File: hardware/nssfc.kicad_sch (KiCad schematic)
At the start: 27 parts, among them U1 STM32F405RGTx, U2 W25Q128JVP, U3 QMC5883P, U4 ICM-20602, U5 BMP580, Y1 25MHz

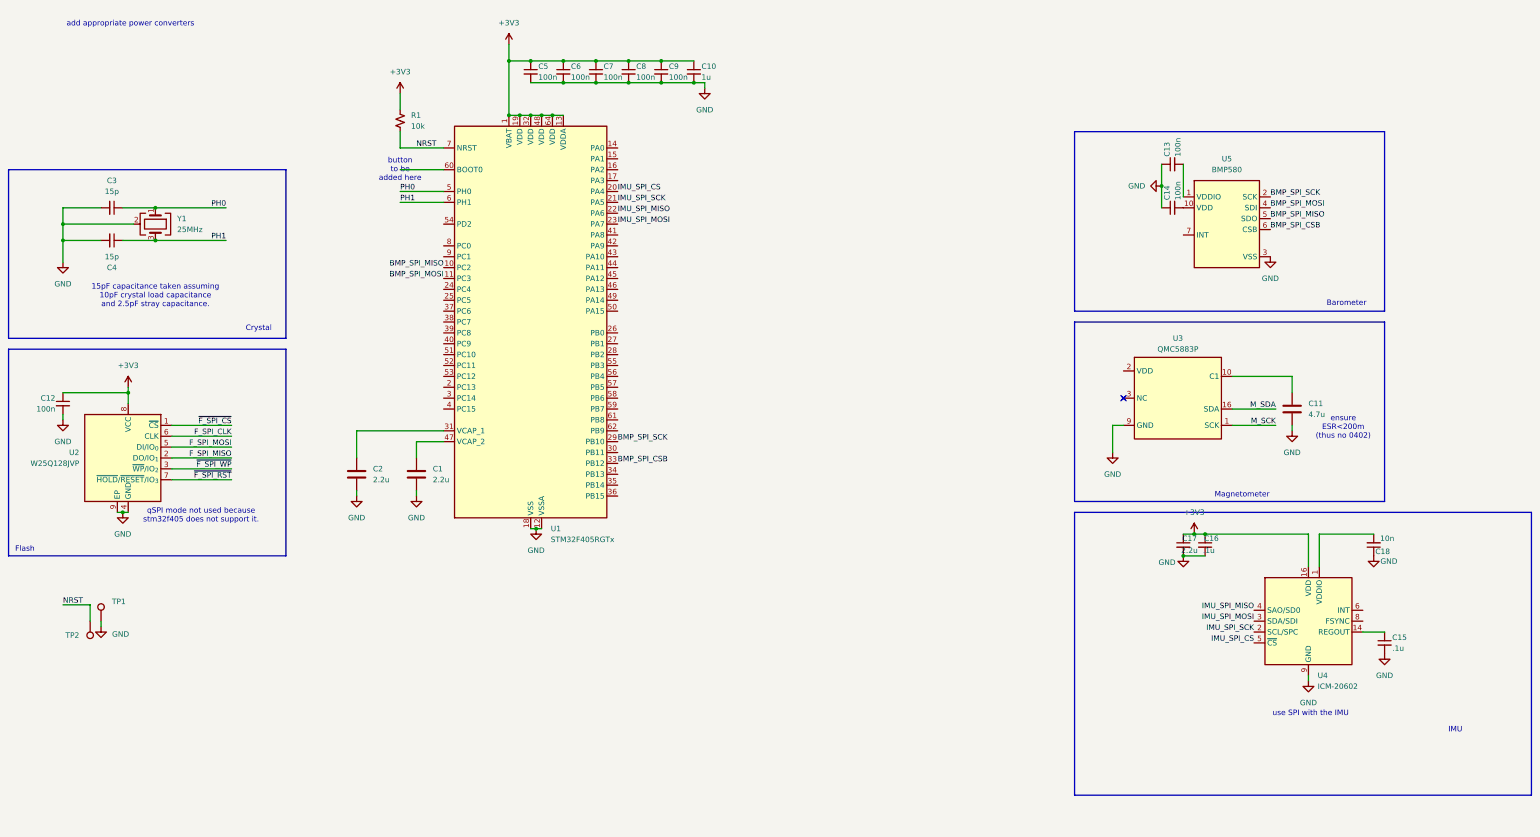
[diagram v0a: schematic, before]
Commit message: worked on the schematic
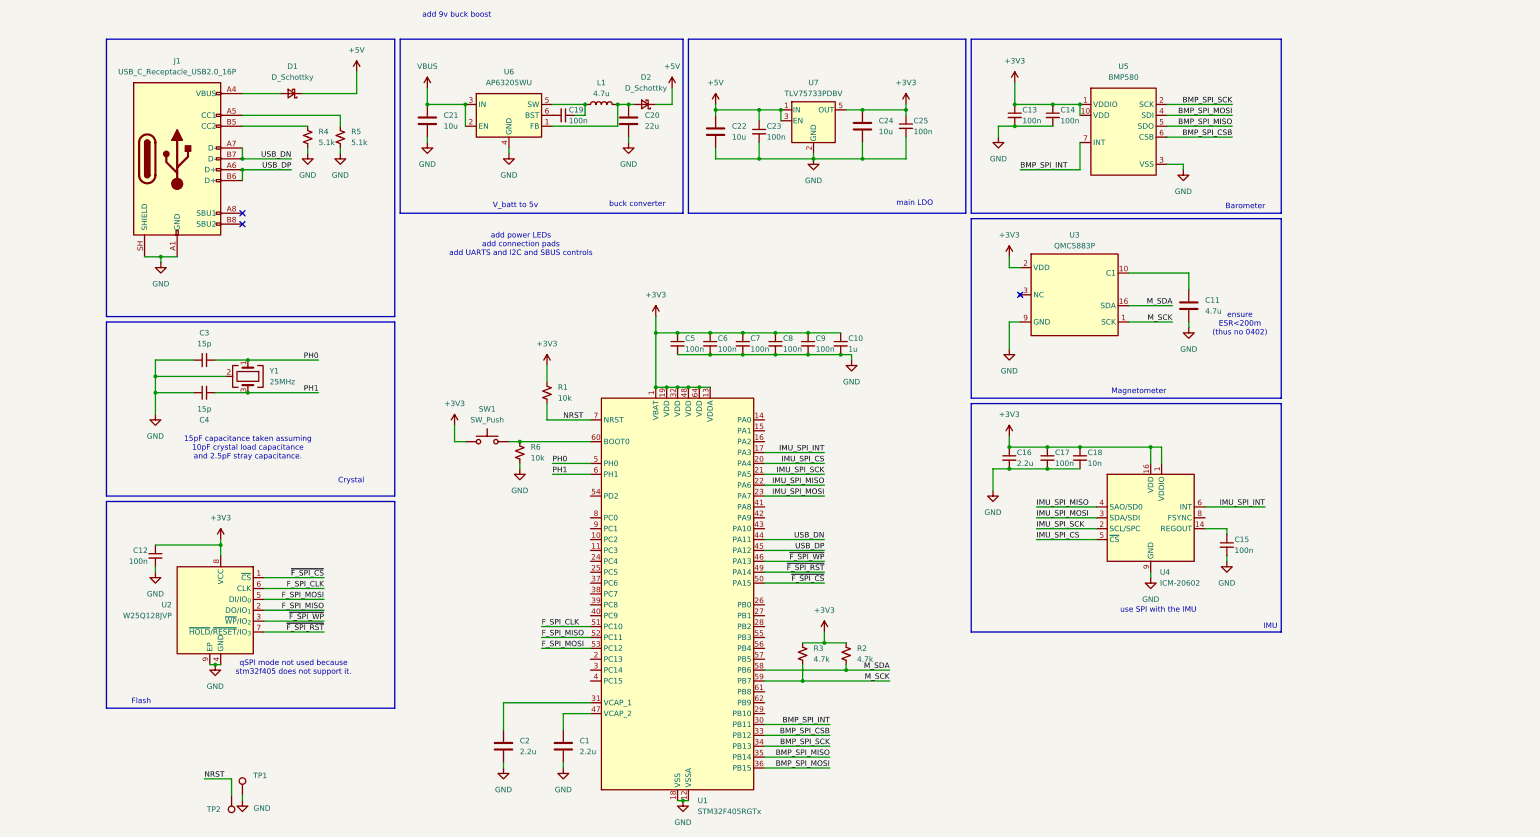
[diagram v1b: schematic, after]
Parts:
- added C19, C23, C25: 100n, Capacitor_SMD:C_0402_1005Metric, symbol Device:C_Small
- added C20: 22u, Capacitor_SMD:C_0805_2012Metric, symbol Device:C
- added C21, C22, C24: 10u, Capacitor_SMD:C_0805_2012Metric, symbol Device:C
- added D1, D2: D_Schottky, Diode_SMD:D_SOD-123F, symbol Device:D_Schottky_Small
- added J1: USB_C_Receptacle_USB2.0_16P, Connector_USB:USB_C_Receptacle_XKB_U262-16XN-4BVC11, symbol Connector:USB_C_Receptacle_USB2.0_16P
- added L1: 4.7u, Inductor_SMD:L_Changjiang_FNR4020S, symbol Device:L
- added R2, R3: 4.7k, Resistor_SMD:R_0402_1005Metric, symbol Device:R_Small_US
- added R4, R5: 5.1k, Resistor_SMD:R_0402_1005Metric, symbol Device:R_Small_US
- added R6: 10k, Resistor_SMD:R_0402_1005Metric, symbol Device:R_Small_US
- added SW1: SW_Push, Button_Switch_SMD:SW_SPST_PTS810, symbol Switch:SW_Push
- added U6: AP63205WU, Package_TO_SOT_SMD:TSOT-23-6, symbol Regulator_Switching:AP63205WU
- added U7: TLV75733PDBV, Package_TO_SOT_SMD:SOT-23-5, symbol Regulator_Linear:TLV75733PDBV
- C1, C10, C12, C13, C14, C18, C2, C3, C4, C5, C6, C7, C8, C9: footprint (none) -> Capacitor_SMD:C_0402_1005Metric
- C11: footprint (none) -> Capacitor_SMD:C_0805_2012Metric
- C15: value .1u -> 100n; footprint (none) -> Capacitor_SMD:C_0402_1005Metric
- C16: value .1u -> 2.2u; footprint (none) -> Capacitor_SMD:C_0402_1005Metric
- C17: value 2.2u -> 100n; footprint (none) -> Capacitor_SMD:C_0402_1005Metric
- R1: footprint (none) -> Resistor_SMD:R_0402_1005Metric
- TP1, TP2: footprint (none) -> TestPoint:TestPoint_Pad_1.0x1.0mm
- Y1: footprint (none) -> Crystal:Crystal_SMD_3225-4Pin_3.2x2.5mm
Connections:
- net +3V3: now also C13.1, C14.1, C18.1, U3.2 (VDD), U4.1 (VDDIO), U5.1 (VDDIO), U5.10 (VDD), C24.1, C25.1, R2.1, R3.1, SW1.1, U7.5 (OUT)
- net BMP_SPI_MISO: now also U1.35 (PB14); no longer U1.10 (PC2)
- net BMP_SPI_MOSI: now also U1.36 (PB15); no longer U1.11 (PC3)
- net BMP_SPI_SCK: now also U1.34 (PB13); no longer U1.29 (PB10)
- net F_SPI_CLK: now also U1.51 (PC10)
- net F_SPI_MISO: now also U1.52 (PC11)
- net F_SPI_MOSI: now also U1.53 (PC12)
- net GND: now also C13.2, C14.2, C18.2, C20.2, C21.2, C22.2, C23.2, C24.2, C25.2, J1.A1 (GND), J1.A12 (GND), J1.B1 (GND), J1.B12 (GND), J1.SH (SHIELD), R4.2, R5.2, R6.2, U6.4 (GND), U7.2 (GND); no longer C13.1, C14.1, C18.1
- net M_SCK: now also U1.59 (PB7), R3.2
- net M_SDA: now also U1.58 (PB6), R2.2
- net ~{F_SPI_CS}: now also U1.50 (PA15)
- net ~{F_SPI_RST}: now also U1.49 (PA14)
- net ~{F_SPI_WP}: now also U1.46 (PA13)
- net IMU_SPI_INT: now reaches U1.17 (PA3)
- net IMU_SPI_INT: now also U4.6 (INT)
- net BMP_SPI_INT: now reaches U1.30 (PB11)
- net BMP_SPI_INT: now also U5.7 (INT)
- net USB_DN: now reaches U1.44 (PA11)
- net USB_DN: now also J1.A7 (D-), J1.B7 (D-)
- net USB_DP: now reaches U1.45 (PA12)
- net USB_DP: now also J1.A6 (D+), J1.B6 (D+)
- net at U1.60 (BOOT0): now also R6.1, SW1.2
- new net: D1.2 (A), J1.A4 (VBUS), J1.A9 (VBUS), J1.B4 (VBUS), J1.B9 (VBUS)
- new net: J1.A5 (CC1), R5.1
- new net: J1.B5 (CC2), R4.1
- new net: C20.1, D2.2 (A), L1.2, U6.1 (FB)
- new net: C19.1, L1.1, U6.5 (SW)
- new net: C19.2, U6.6 (BST)
- new net +5V: C22.1, C23.1, D1.1 (K), D2.1 (K), U7.1 (IN), U7.3 (EN)
- new net VBUS: C21.1, U6.2 (EN), U6.3 (IN)
- no-connect marks 1 -> 3
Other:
- note added: "V_batt to 5v"
- note added: "add 9v buck boost"
- note added: "add power LEDs add connection pads add UARTS and I2C and SBUS controls"
- note added: "buck converter"
- note added: "main LDO"
- note removed: "add appropriate power converters"
- note removed: "button to be added here"
- moved on the sheet: C1, C10, C11, C12, C15, C2, C3, C4, C5, C6, C7, C8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
